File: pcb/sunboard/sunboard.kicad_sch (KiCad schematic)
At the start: 154 parts, among them SW1 SW_Push_LED, SW10 SW_Push_LED, SW100 SW_Push_LED, SW101 SW_Push_LED, SW102 SW_Push_LED, SW103 SW_Push_LED, SW104 SW_Push_LED, SW105 SW_Push_LED, SW106 SW_Push_LED, SW107 SW_Push_LED, SW108 SW_Push_LED, SW109 SW_Push_LED, SW11 SW_Push_LED, SW110 SW_Push_LED, SW111 SW_Push_LED, SW112 SW_Push_LED, SW113 SW_Push_LED, SW114 SW_Push_LED, SW115 SW_Push_LED, SW116 SW_Push_LED, SW117 SW_Push_LED, SW118 SW_Push_LED, SW119 SW_Push_LED, SW12 SW_Push_LED, SW120 SW_Push_LED, SW121 SW_Push_LED, SW122 SW_Push_LED, SW123 SW_Push_LED, SW124 SW_Push_LED, SW125 SW_Push_LED, SW126 SW_Push_LED, SW127 SW_Push_LED, SW128 SW_Push_LED, SW129 SW_Push_LED, SW13 SW_Push_LED, SW130 SW_Push_LED, SW131 SW_Push_LED, SW132 SW_Push_LED, SW133 SW_Push_LED, SW134 SW_Push_LED, SW135 SW_Push_LED, SW136 SW_Push_LED, SW137 SW_Push_LED, SW138 SW_Push_LED, SW139 SW_Push_LED, SW14 SW_Push_LED, SW140 SW_Push_LED, SW141 SW_Push_LED, SW142 SW_Push_LED, SW143 SW_Push_LED, SW144 SW_Push_LED, SW145 SW_Push_LED, SW146 SW_Push_LED, SW147 SW_Push_LED, SW148 SW_Push_LED, SW149 SW_Push_LED, SW15 SW_Push_LED, SW150 SW_Push_LED, SW151 SW_Push_LED, SW152 SW_Push_LED, SW153 SW_Push_LED, SW154 SW_Push_LED, SW16 SW_Push_LED, SW17 SW_Push_LED, SW18 SW_Push_LED, SW19 SW_Push_LED, SW2 SW_Push_LED, SW20 SW_Push_LED, SW21 SW_Push_LED, SW22 SW_Push_LED, SW23 SW_Push_LED, SW24 SW_Push_LED, SW25 SW_Push_LED, SW26 SW_Push_LED, SW27 SW_Push_LED, SW28 SW_Push_LED, SW29 SW_Push_LED, SW3 SW_Push_LED, SW30 SW_Push_LED, SW31 SW_Push_LED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

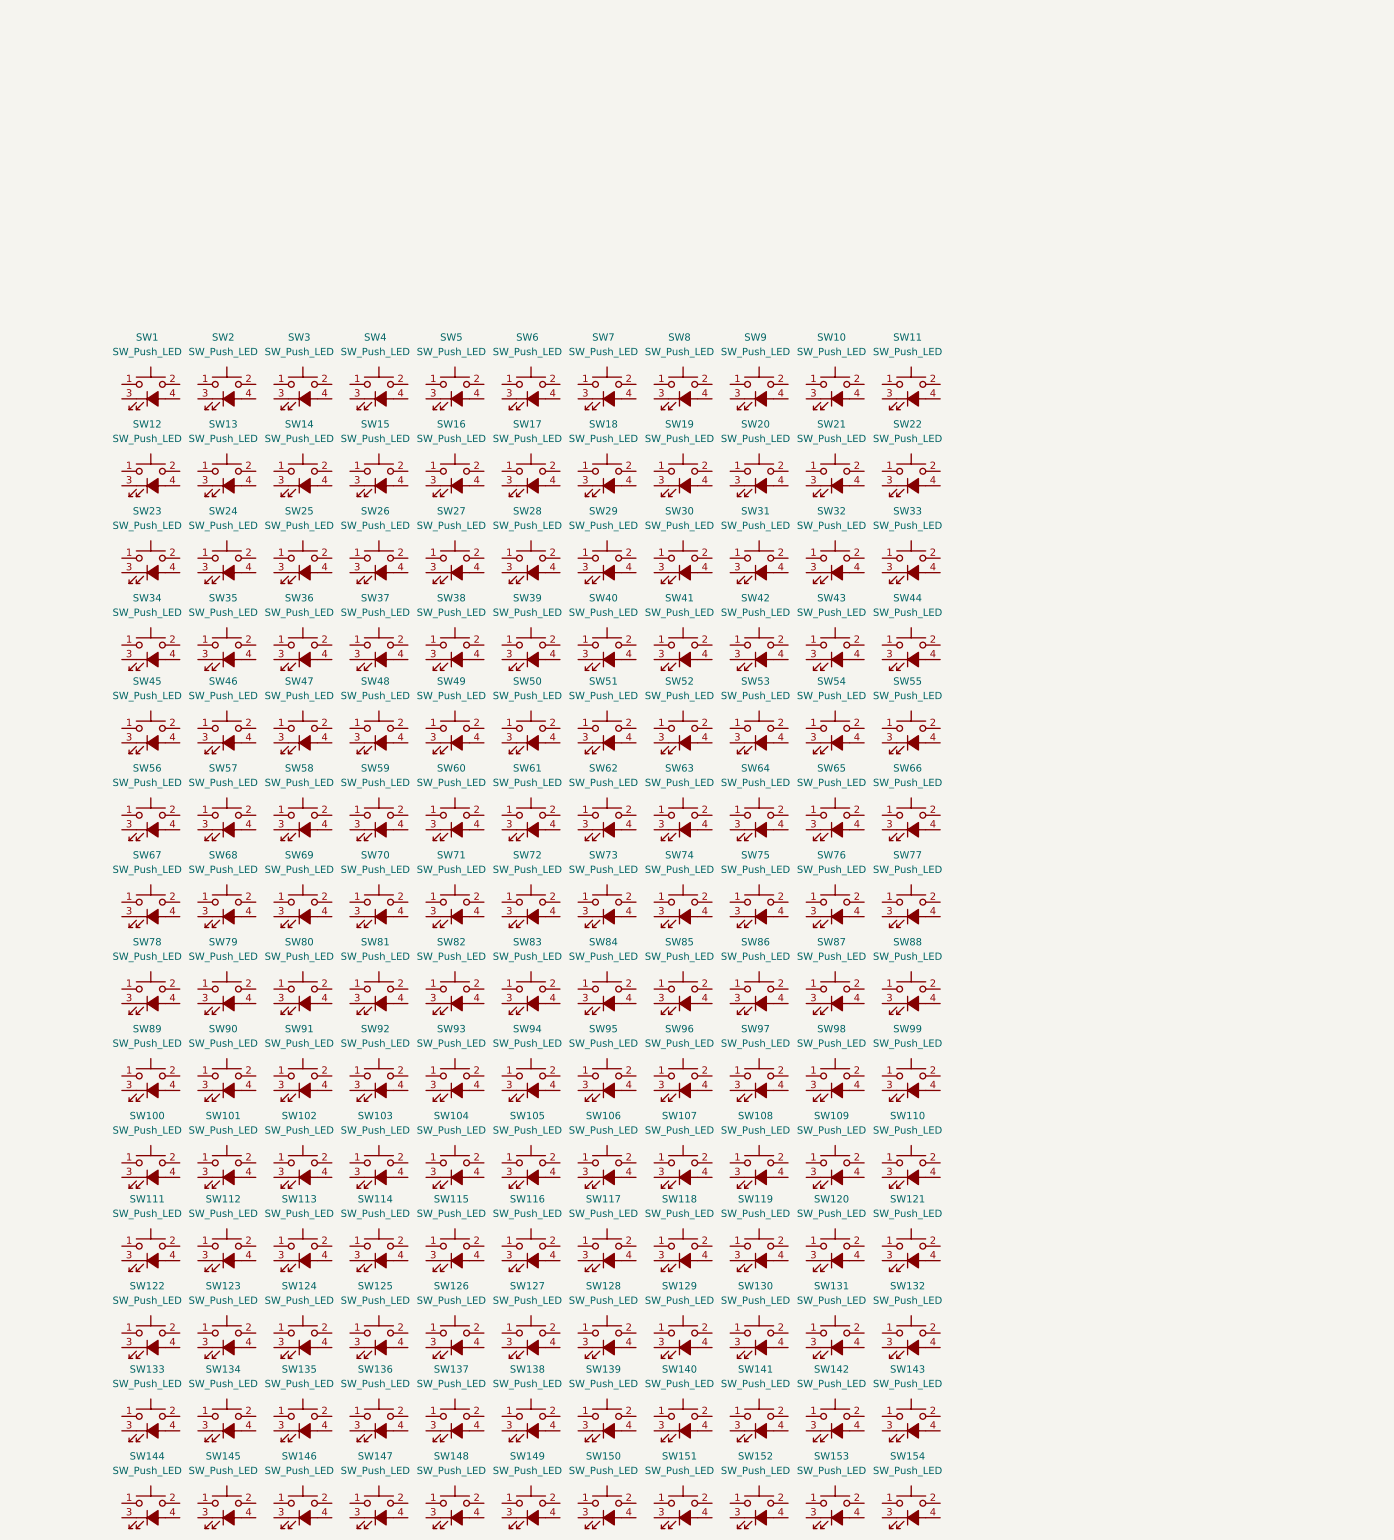
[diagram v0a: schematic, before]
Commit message: feat: get basic POC for 8x8 out
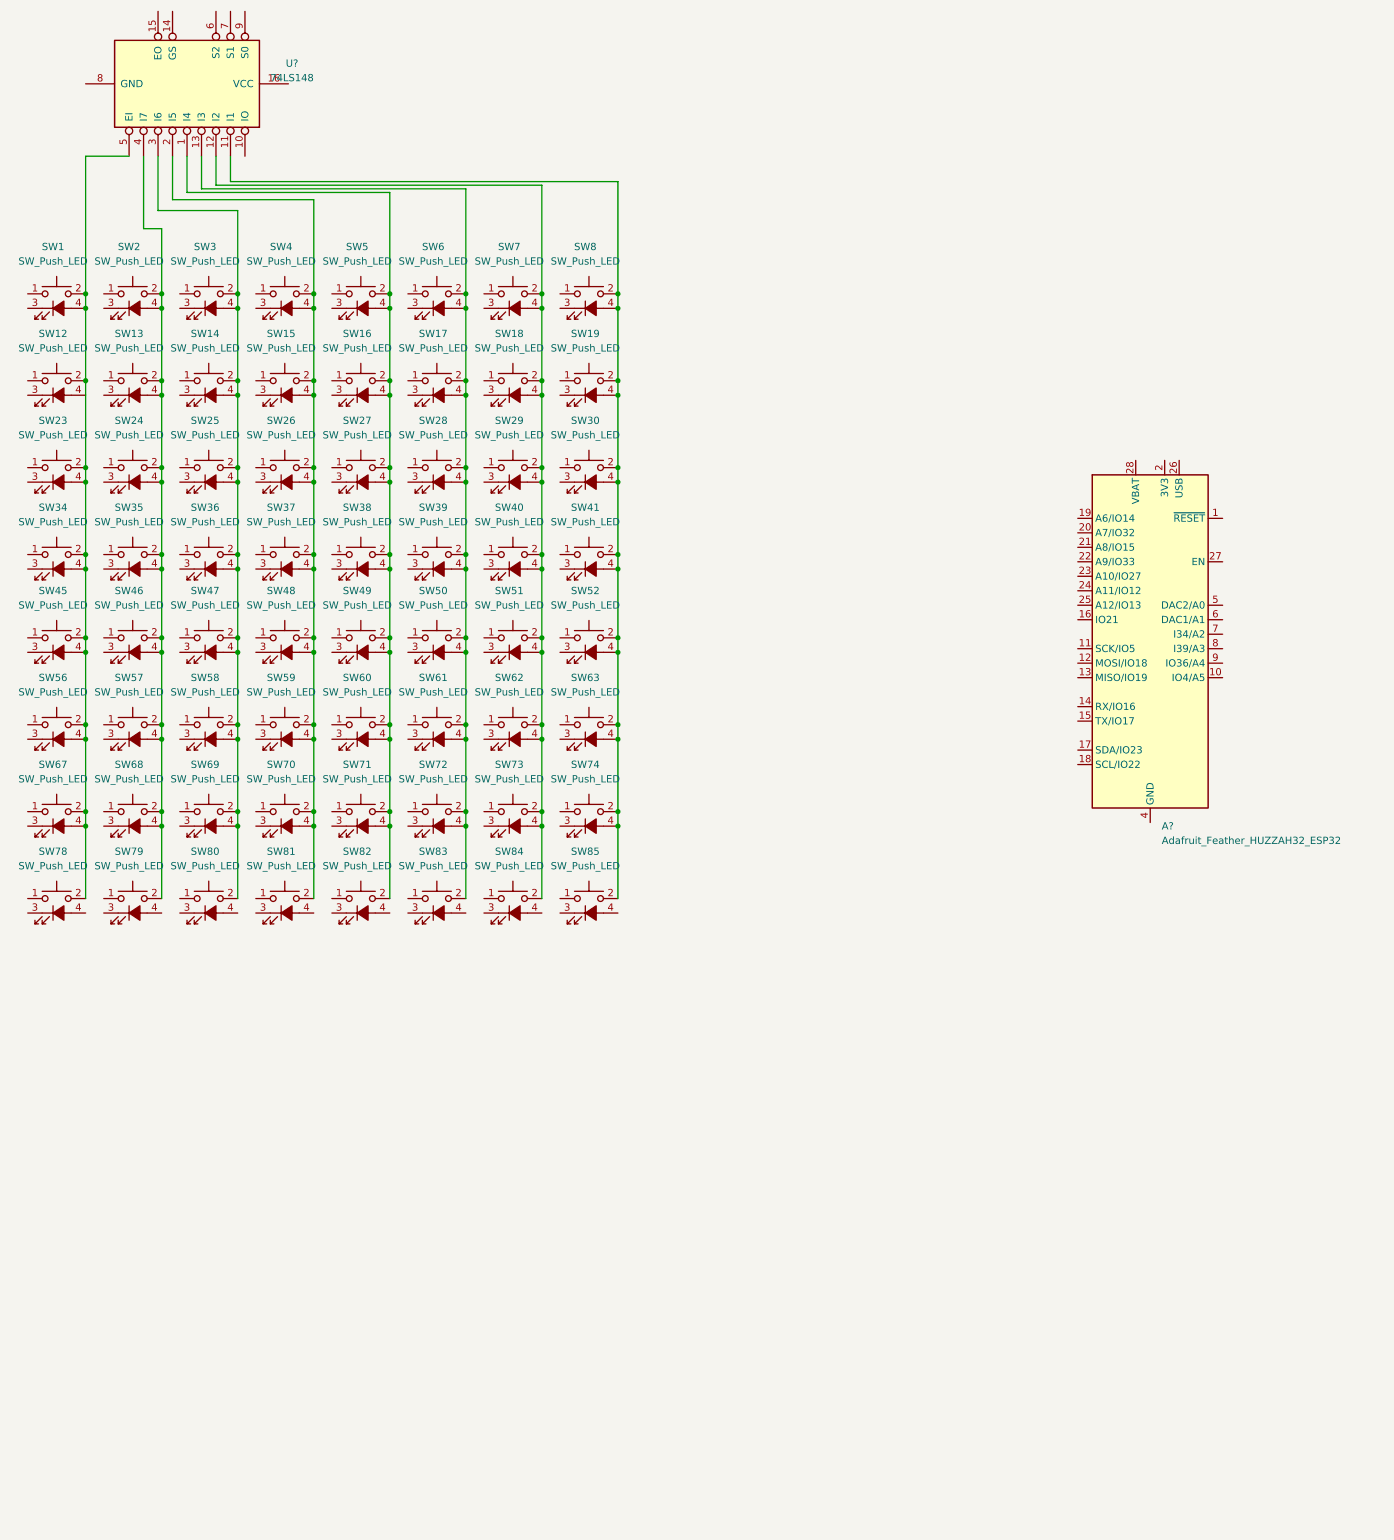
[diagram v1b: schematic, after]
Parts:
- removed SW10, SW100, SW101, SW102, SW103, SW104, SW105, SW106, SW107, SW108, SW109, SW11, SW110, SW111, SW112, SW113, SW114, SW115, SW116, SW117, SW118, SW119, SW120, SW121, SW122, SW123, SW124, SW125, SW126, SW127, SW128, SW129, SW130, SW131, SW132, SW133, SW134, SW135, SW136, SW137, SW138, SW139, SW140, SW141, SW142, SW143, SW144, SW145, SW146, SW147, SW148, SW149, SW150, SW151, SW152, SW153, SW154, SW20, SW21, SW22, SW31, SW32, SW33, SW42, SW43, SW44, SW53, SW54, SW55, SW64, SW65, SW66, SW75, SW76, SW77, SW86, SW87, SW88, SW89, SW9, SW90, SW91, SW92, SW93, SW94, SW95, SW96, SW97, SW98, SW99: SW_Push_LED, symbol Switch:SW_Push_LED
- added A?: Adafruit_Feather_HUZZAH32_ESP32, Module:Adafruit_Feather, symbol MCU_Module:Adafruit_Feather_HUZZAH32_ESP32
- added U?: 74LS148, symbol 74xx:74LS148
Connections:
- net at SW74.2: now also SW19.2, SW19.4 (A), SW30.2, SW30.4 (A), SW41.2, SW41.4 (A), SW52.2, SW52.4 (A), SW63.2, SW63.4 (A), SW74.4 (A), SW8.2, SW8.4 (A), SW85.2, U?.11 (I1)
- net at SW70.2: now also SW15.2, SW15.4 (A), SW26.2, SW26.4 (A), SW37.2, SW37.4 (A), SW4.2, SW4.4 (A), SW48.2, SW48.4 (A), SW59.2, SW59.4 (A), SW70.4 (A), SW81.2, U?.2 (I5)
- net at SW72.2: now also SW17.2, SW17.4 (A), SW28.2, SW28.4 (A), SW39.2, SW39.4 (A), SW50.2, SW50.4 (A), SW6.2, SW6.4 (A), SW61.2, SW61.4 (A), SW72.4 (A), SW83.2, U?.13 (I3)
- net at SW24.2: now also SW13.2, SW13.4 (A), SW2.2, SW2.4 (A), SW24.4 (A), SW35.2, SW35.4 (A), SW46.2, SW46.4 (A), SW57.2, SW57.4 (A), SW68.2, SW68.4 (A), SW79.2, U?.4 (I7)
- net at SW45.2: now also SW1.2, SW1.4 (A), SW12.2, SW23.2, SW23.4 (A), SW34.2, SW34.4 (A), SW45.4 (A), SW56.2, SW56.4 (A), SW67.2, SW67.4 (A), SW78.2, U?.5 (EI)
- net at SW62.2: now also SW18.2, SW18.4 (A), SW29.2, SW29.4 (A), SW40.2, SW40.4 (A), SW51.2, SW51.4 (A), SW62.4 (A), SW7.2, SW7.4 (A), SW73.2, SW73.4 (A), SW84.2, U?.12 (I2)
- net at SW25.2: now also SW14.2, SW14.4 (A), SW25.4 (A), SW3.2, SW3.4 (A), SW36.2, SW36.4 (A), SW47.2, SW47.4 (A), SW58.2, SW58.4 (A), SW69.2, SW69.4 (A), SW80.2, U?.3 (I6)
- net at SW60.2: now also SW16.2, SW16.4 (A), SW27.2, SW27.4 (A), SW38.2, SW38.4 (A), SW49.2, SW49.4 (A), SW5.2, SW5.4 (A), SW60.4 (A), SW71.2, SW71.4 (A), SW82.2, U?.1 (I4)
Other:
- moved on the sheet: SW1, SW12, SW13, SW14, SW15, SW16, SW17, SW18, SW19, SW2, SW23, SW24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
